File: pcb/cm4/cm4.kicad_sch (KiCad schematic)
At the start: 0 parts

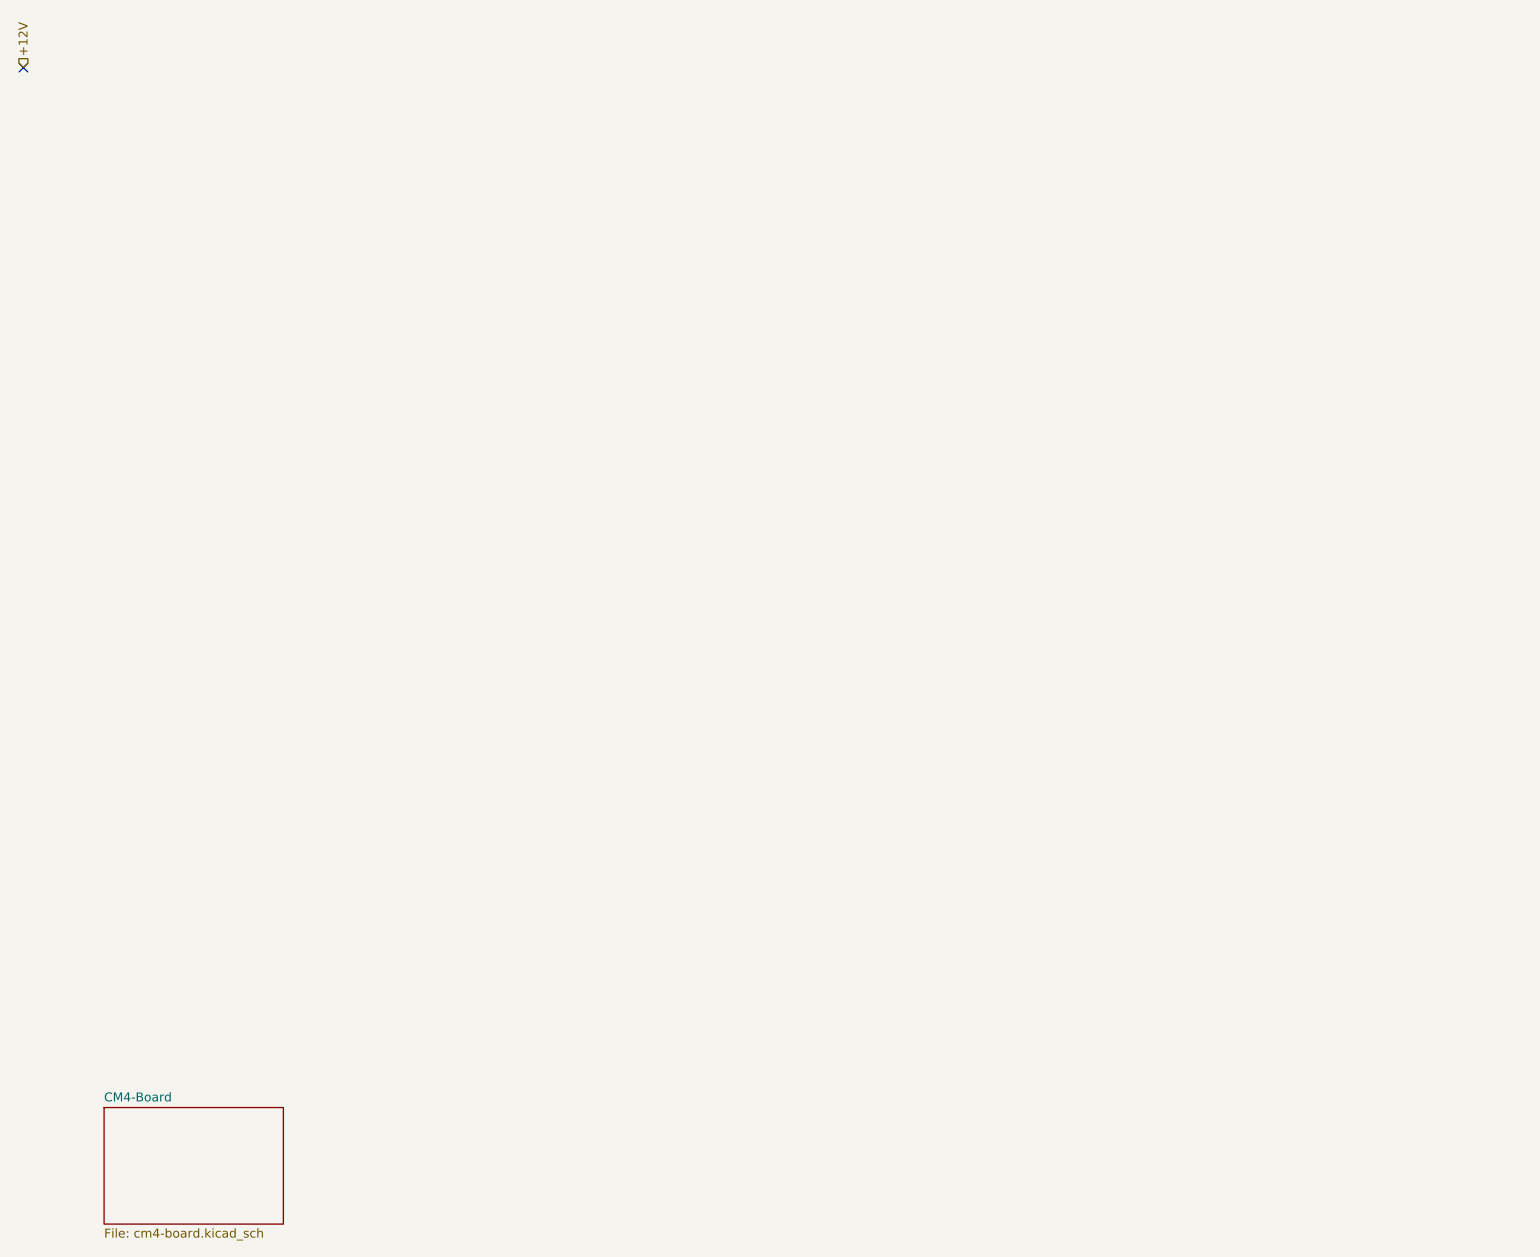
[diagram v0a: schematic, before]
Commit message: update cm4 board
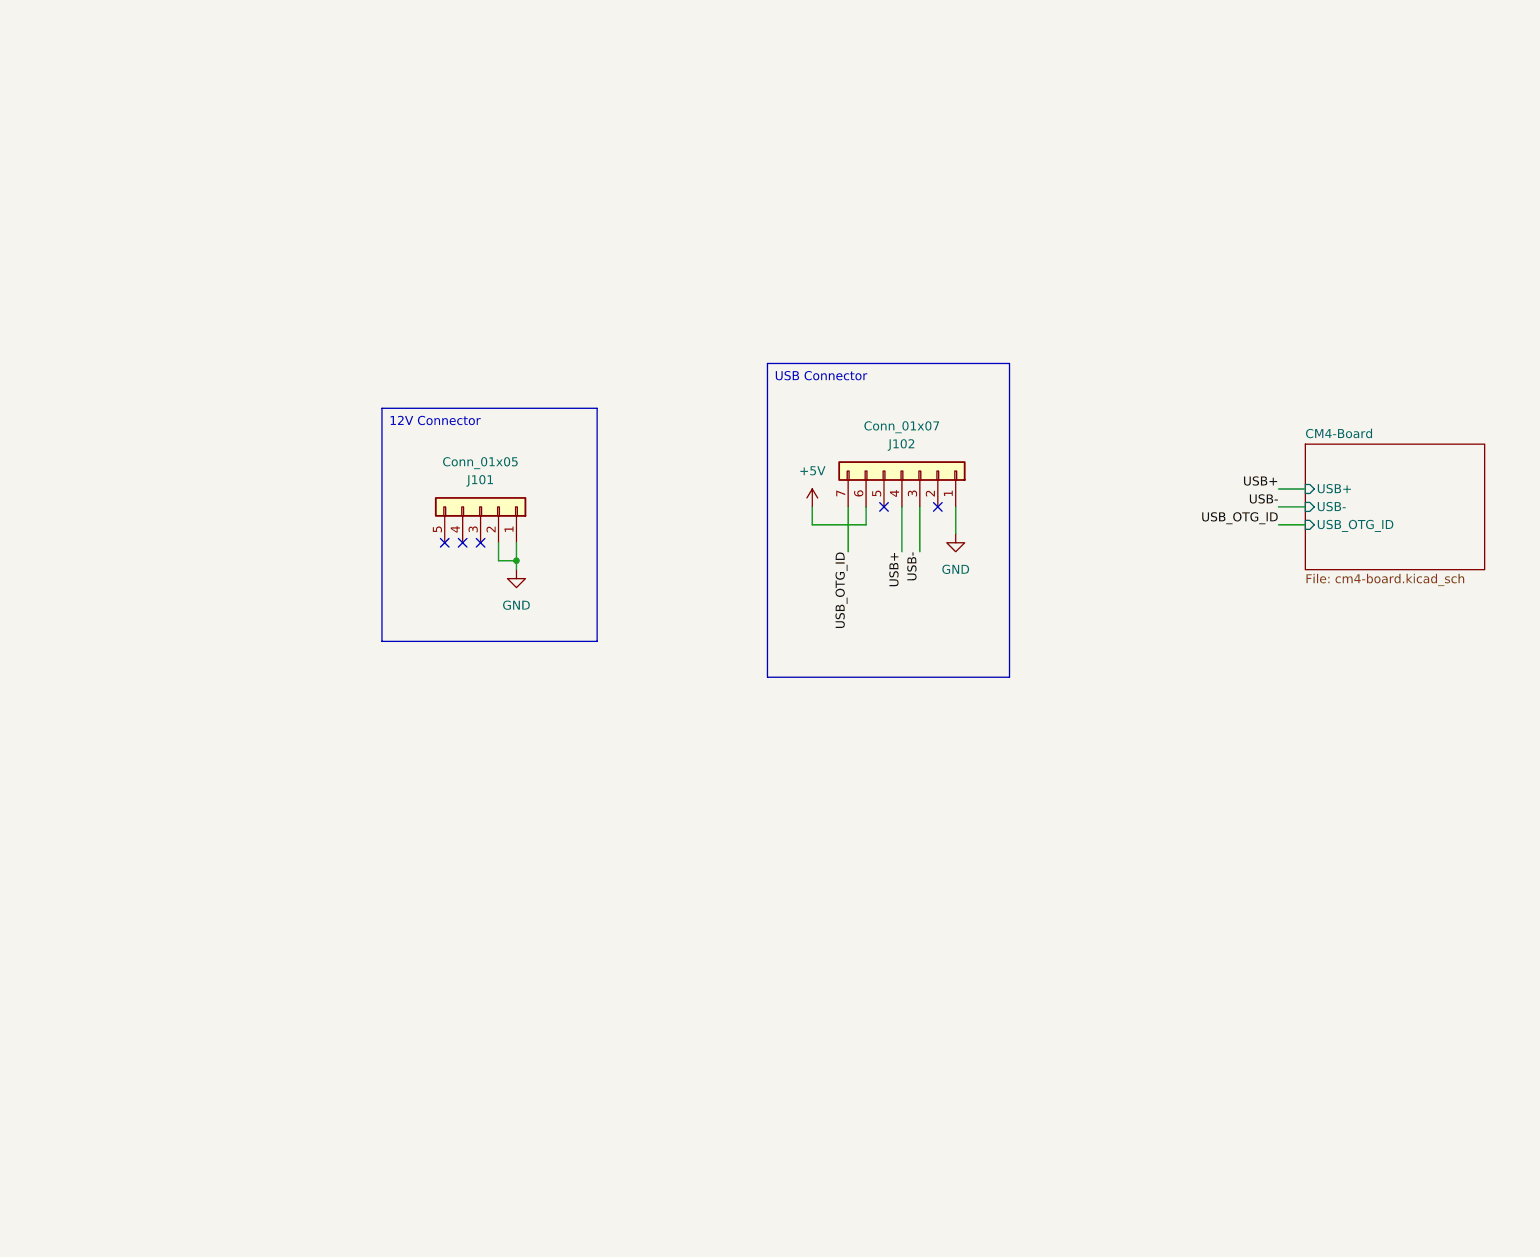
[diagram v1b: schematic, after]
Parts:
- added J101: Conn_01x05, symbol Connector_Generic:Conn_01x05
- added J102: Conn_01x07, symbol Connector_Generic:Conn_01x07
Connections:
- new net +5V: J102.6 (Pin_6)
- new net GND: J101.1 (Pin_1), J101.2 (Pin_2), J102.1 (Pin_1)
- new net USB+: J102.4 (Pin_4)
- new net USB-: J102.3 (Pin_3)
- new net USB_OTG_ID: J102.7 (Pin_7)
- no-connect marks 1 -> 5
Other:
- sheet CM4-Board ports: added USB+, USB-, USB_OTG_ID; removed none
- title: CM4 -> Bus Connector
